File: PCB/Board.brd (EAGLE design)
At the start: 74.1 x 78.9 mm, 32 parts, among them K1 G5LE, K2 G5LE, K3 G5LE, Q1 MOSFET-NCHANNELSMD, Q2 MOSFET-NCHANNELSMD, Q3 MOSFET-NCHANNELSMD

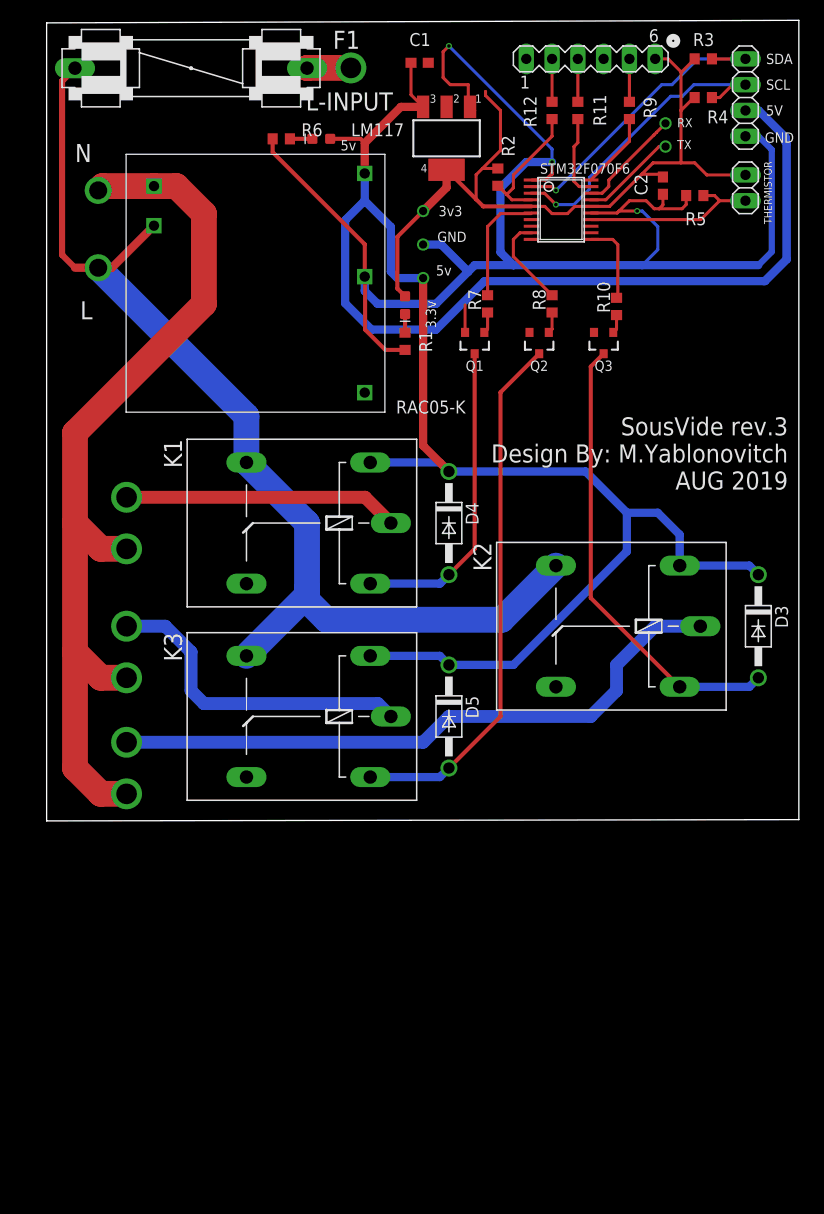
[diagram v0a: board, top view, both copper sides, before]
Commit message: v2
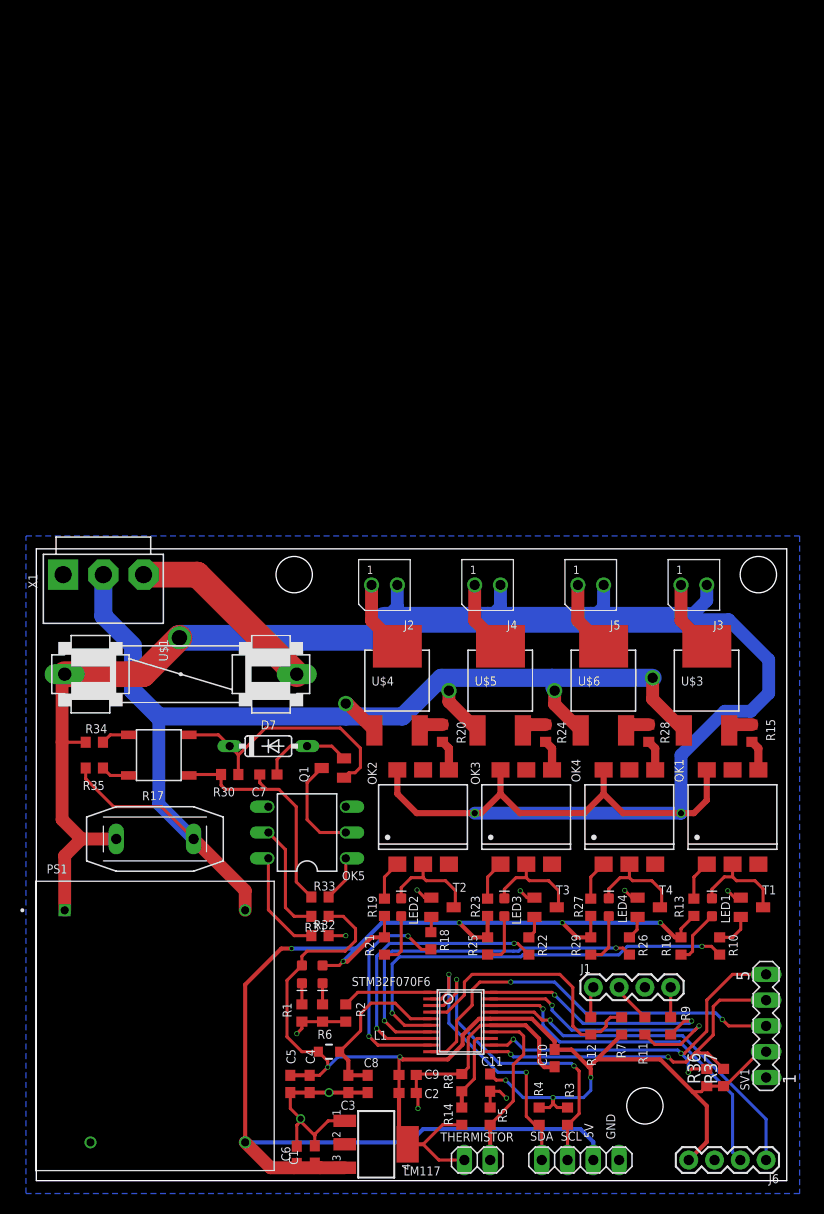
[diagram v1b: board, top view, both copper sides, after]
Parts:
- removed D3, D4, D5: 1N4004, diode:DO41-10
- removed K1, K2, K3: G5LE, relay:G5LE
- removed Q2, Q3: MOSFET-NCHANNELSMD, fets:SOT23-3
- removed RAC05-K: AC/DC-CONVERTER, SousVide Library:AC/DC-CONVERTER
- removed SV2: (no value), con-lstb:MA06-1
- added C10, C5, C8: 1u, rcl:C0603
- added C11, C9: 2.2uF, rcl:C0603
- added C3, C4: 0.1u, rcl:C0603
- added C6: 10u, rcl:C0603
- added C7: 44u, rcl:C0603
- added D7: 1N4148DO35-7, diode:DO35-7
- added J1, J6: (no value), SparkFun-Connectors:1X04
- added J2, J3, J4, J5: (no value), Wurth_Elektronik_Electromechanic_Wire_to_Board_Connectors_rev19a:66100211622
- added L1: 40Ohm@100MHz, Wurth_EMC Components_WE-CBF:WE-CBF_0805(W=3.0)
- added LED1, LED2, LED3, LED4: Yellow, SparkFun-LED:LED-0603
- added OK1, OK2, OK3, OK4: MOC3031S, optocoupler:DIL6-SMD
- added OK5: 4N35, optocoupler:DIL06
- added PS1: RAC03-05SK, SousVide Library:CONV_RAC03-05SK
- added R13, R19, R23, R27: 2k, rcl:R0603
- added R14: 1k5, rcl:R0603
- added R15, R20, R28: 250, rcl:R0603
- added R16, R21, R25, R29, R36, R37: 1k, rcl:R0603
- added R17: P594, varistor:P594
- added R18, R22, R26: 500r, rcl:R0603
- added R24: 24k, rcl:R0603
- added R30: 5k, rcl:R0603
- added R31: 10k, rcl:R0603
- added R32: 100k, rcl:R0603
- added R33: 330r, rcl:R0603
- added R34, R35: 50k, rcl:R0603
- added SV1: (no value), con-lstb:MA05-1
- added T1, T2, T3, T4: (no value), transistor:SOT23-EBC
- added U$1: MDB8S, SousVide Library:4-MICRODIP
- added U$3, U$4, U$5, U$6: SST04K-800SW, SousVide Library:DPAK
- added X1: B3P-VH, con-JST VH:B3P-VH
- Q1: value MOSFET-NCHANNELSMD -> BC847SMD; device fets:SOT23-3 -> SousVide Library:SOT23
- R10: value 250 -> 500r
- R2: value 3k3 -> 10k
- R7: value 250 -> 10k
- R8: value 250 -> 1k5
- moved C1 108.0 mm to (27.4, 2.58), turned to 90 degrees
- moved JP1 105.9 mm to (53.6, 2.03), turned to 0 degrees
- moved R3 105.4 mm to (49.5, 6.35), turned to 270 degrees
- moved R4 101.2 mm to (52.3, 6.35), turned to 270 degrees
- moved THERMISTOR 99.3 mm to (43.4, 2.03), turned to 0 degrees
- moved LM117 99.3 mm to (33.5, 3.58), turned to 270 degrees
- moved R5 92.9 mm to (44.7, 6.35), turned to 90 degrees
- moved C2 92.8 mm to (36.6, 8.64), turned to 0 degrees
- moved R11 90.4 mm to (59.9, 15.2)
- moved R9 90.3 mm to (62.5, 15.2)
- moved R12 90.3 mm to (54.6, 15.2)
- moved R6 86.2 mm to (28.2, 16.5), turned to 270 degrees
- moved R2 83.7 mm to (30.5, 16.5)
- moved D2 82.3 mm to (28.2, 20.3), turned to 270 degrees
- moved STM32F070F6 80.6 mm to (41.8, 15.6)
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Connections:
- removed net GND: C1.2, C2.2, JP1.4, LM117.1, R1.2, R5.2, R6.2, RAC05-K.GND, STM32F070F6.1, STM32F070F6.15, SV2.4
- removed net N$6: D5.A, K3.2, Q2.3
- removed net RELAY1: R7.2, STM32F070F6.6
- removed net RELAY2: R8.2, STM32F070F6.9
- removed net RELAY3: R10.2, STM32F070F6.11
- removed net SWO: SV2.1
- removed net VAC(L): F1.2, K1.S, K2.S, K3.S, RAC05-K.L
- removed net VAC(L)-OUTPUT1: K1.P
- removed net VAC(L)-OUTPUT2: K3.P
- removed net VAC(L)-OUTPUT3: K2.P
- removed net VAC(N): RAC05-K.N
- new net CTRL1: R18.2, STM32F070F6.9
- new net CTRL2: R22.2, STM32F070F6.8
- new net CTRL3: R26.2, STM32F070F6.7
- new net CTRL4: R10.2, STM32F070F6.6
- new net ENCODER_A: R36.2, STM32F070F6.12, SV1.5
- new net ENCODER_B: R37.2, STM32F070F6.11, SV1.4
- new net ENCODER_BUTTON: STM32F070F6.10, SV1.3
- new net FET4: R26.1, T4.B
- new net N$10: LED1.A, R16.2
- new net N$11: J3.1, U$3.4
- new net N$12: OK2.1, R19.1
- new net N$13: OK2.4, R20.2
- new net N$14: R20.1, U$4.3
- new net N$15: LED2.A, R21.2
- new net N$16: J2.1, U$4.4
- new net N$17: LED3.C, OK3.2, T3.C
- new net N$18: OK3.1, R23.1
- new net N$20: OK3.4, R24.2
- new net N$23: R24.1, U$5.3
- new net N$24: LED3.A, R25.2
- new net N$25: J4.1, U$5.4
- new net N$26: LED4.C, OK4.2, T4.C
- new net N$27: OK4.1, R27.1
- new net N$28: OK4.4, R28.2
- new net N$29: R28.1, U$6.3
- new net N$30: LED4.A, R29.2
- new net N$31: J5.1, U$6.4
- new net N$32: D7.C, Q1.1, R30.2, U$1.4
- new net N$33: C7.1, R30.1, R33.1, U$1.3
- new net N$34: C7.2, D7.A, Q1.2
- new net N$35: OK5.2, Q1.3
- new net N$36: OK5.6, R32.1
- new net N$37: OK5.1, R33.2
- new net N$38: R34.2, U$1.1
- new net N$39: R35.2, U$1.2
- new net N$43: R2.2, STM32F070F6.1
- new net N$5: LED1.C, OK1.2, T1.C
- new net N$7: OK1.4, R15.2
- new net N$8: OK1.1, R13.1
- new net N$9: R15.1, U$3.3
- new net THERM-CALIBRATE: R14.2, R8.1, STM32F070F6.13
- new net V+: F1.2, J2.2, J3.2, J4.2, J5.2, OK1.6, OK2.6, OK3.6, OK4.6, PS1.1, R17.2, R34.1
- new net V-: PS1.4, R17.1, R35.1, U$3.1, U$4.1, U$5.1, U$6.1, X1.2
- new net ZERO-CROSS-DETECT: OK5.5, R31.2
- net +3V3: now also C10.1, C11.1, C4.1, C5.1, C9.1, J6.4, L1.1, R14.1, R31.1, R36.1, R37.1, R7.1, SV1.2; no longer R2.2, STM32F070F6.5, SV2.6
- net +5V: now also C6.1, PS1.3, R13.2, R16.1, R19.2, R21.1, R23.2, R25.1, R27.2, R29.1; no longer D3.C, D4.C, D5.C, K1.1, K2.1, K3.1, RAC05-K.+5V
- net FET1: now also R18.1, T2.B; no longer Q1.1, R7.1
- net FET2: now also R22.1, T3.B; no longer Q2.1, R8.1
- net FET3: now also T1.B; no longer Q3.1
- net N$19: now also J1.4; no longer SV2.5
- net N$21: now also J1.2; no longer SV2.3
- net N$22: now also J1.1; no longer SV2.2
- net N$3: now also C3.1, C8.1, L1.2, STM32F070F6.5; no longer D4.A, K1.2, Q1.3
- net N$4: now also LED2.C, OK2.2, T2.C; no longer D3.A, K2.2, Q3.3
- net NRST: now also R7.2; no longer R2.1
- net PE: now also C1.2, C10.2, C11.2, C2.2, C3.2, C4.2, C5.2, C6.2, C8.2, C9.2, J1.3, J6.3, JP1.4, LM117.1, OK5.4, PS1.2, R1.2, R2.1, R32.2, R5.2, R6.2, R8.2, STM32F070F6.15, SV1.1, T1.E, T2.E, T3.E, T4.E, X1.1; no longer Q1.2, Q2.2, Q3.2
- net RX: now also J6.2
- net TX: now also J6.1
- net VAC(L)-INPUT: now also X1.3
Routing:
- net V+: track 0.00 -> 205.4 mm, vias 0 -> 3
- net GND: track 154.6 -> 0.00 mm, vias 4 -> 0
- net VAC(L): track 141.1 -> 0.00 mm, vias 1 -> 0
- net V-: track 0.00 -> 127.9 mm, vias 0 -> 4
- net VAC(N): track 90.0 -> 0.00 mm, vias 4 -> 0
- net +5V: track 222.1 -> 135.6 mm, vias 1 -> 5
- net VAC(L)-OUTPUT3: track 62.7 -> 0.00 mm, vias 1 -> 0
- net PE: track 2.71 -> 61.3 mm, vias 0 -> 10
- net N$6: track 52.6 -> 0.00 mm
- net +3V3: track 80.3 -> 129.2 mm, vias 1 -> 5
- net CTRL4: track 0.00 -> 42.5 mm, vias 0 -> 2
- net ENCODER_BUTTON: track 0.00 -> 39.7 mm, vias 0 -> 2
- net ENCODER_A: track 0.00 -> 37.1 mm, vias 0 -> 3
- net CTRL3: track 0.00 -> 36.0 mm, vias 0 -> 2
- net ENCODER_B: track 0.00 -> 35.2 mm, vias 0 -> 2
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- added copper zone on layer 16, net PE
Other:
- board size 74.1 x 78.9 mm -> 73.9 x 62.2 mm
- board text added: "SousVide rev 3 by M.Yablonovitch JUL 2020"
- board text removed: "3.3v"
- board text removed: "3v3"
- board text removed: "5v"
- board text removed: "L"
- board text removed: "L-INPUT"
- board text removed: "N"
- board text removed: "RX"
- board text removed: "SousVide rev.3 Design By: M.Yablonovitch AUG 2019"
- board text removed: "TX"
